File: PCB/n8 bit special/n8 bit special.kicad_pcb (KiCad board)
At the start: 4 copper layers, 99.9 x 100 mm, 50 parts, among them J1 USB_B_Micro, J2 PORT0, J3 PORT2, J4 PORT1, J6 Conn_02x08_Odd_Even, Q1 2N3904, SW1 SW_Push_Dual, U1 W65C02SxP, U10 74HC00, U2 CY62256-70PC, U3 CY62256-70PC, U4 28C256, U5 74LS21, U6 22V10C, U7 DS1813, U8 SC28L92_PLC44, U9 FT230XS, X1 3.6864Mhz

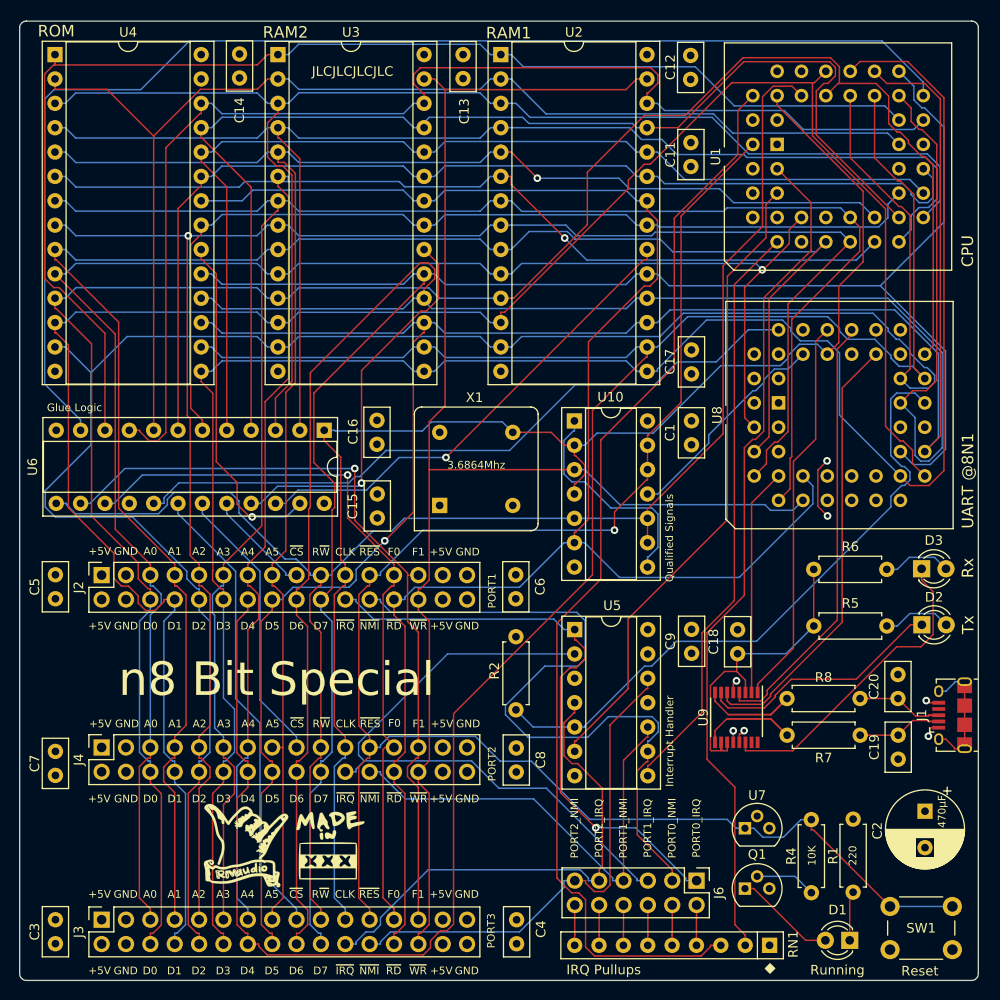
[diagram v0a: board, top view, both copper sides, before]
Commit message: release candidate for v2
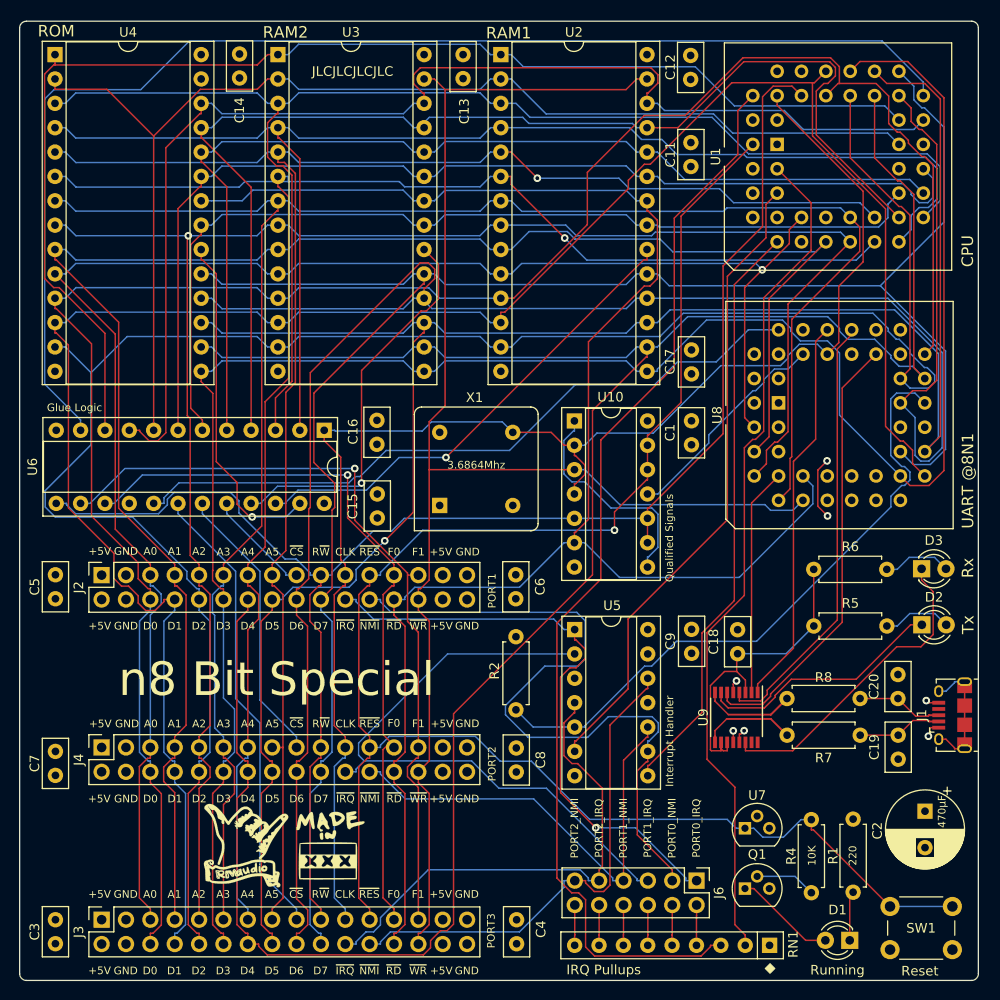
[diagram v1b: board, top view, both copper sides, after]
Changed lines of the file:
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@@
-(kicad_pcb (version 20171130) (host pcbnew "(5.1.9-0-10_14)")
+(kicad_pcb (version 20171130) (host pcbnew "(5.1.12-1-10_14)")
   (general
     (thickness 1.6)
@@
     )
   )
+  (gr_text GND (at 133.60908 130.90652) (layer F.SilkS)
+    (effects (font (size 0.8 0.8) (thickness 0.15)))
+  )
+  (gr_text ~RES (at 123.44908 130.90652) (layer F.SilkS)
+    (effects (font (size 0.8 0.8) (thickness 0.15)))
+  )
+  (gr_text +5V (at 130.89128 130.89382) (layer F.SilkS)
+    (effects (font (size 0.8 0.8) (thickness 0.15)))
+  )
+  (gr_text R~W (at 118.36908 130.90652) (layer F.SilkS)
+    (effects (font (size 0.8 0.8) (thickness 0.15)))
+  )
+  (gr_text A0 (at 100.58908 130.90652) (layer F.SilkS)
+    (effects (font (size 0.8 0.8) (thickness 0.15)))
+  )
+  (gr_text GND (at 98.04908 130.90652) (layer F.SilkS)
+    (effects (font (size 0.8 0.8) (thickness 0.15)))
+  )
+  (gr_text A2 (at 105.66908 130.90652) (layer F.SilkS)
+    (effects (font (size 0.8 0.8) (thickness 0.15)))
+  )
+  (gr_text +5V (at 95.33128 130.90652) (layer F.SilkS)
+    (effects (font (size 0.8 0.8) (thickness 0.15)))
+  )
+  (gr_text A1 (at 103.12908 130.90652) (layer F.SilkS)
+    (effects (font (size 0.8 0.8) (thickness 0.15)))
+  )
+  (gr_text F1 (at 128.52908 130.90652) (layer F.SilkS)
+    (effects (font (size 0.8 0.8) (thickness 0.15)))
+  )
+  (gr_text CLK (at 120.90908 130.90652) (layer F.SilkS)
+    (effects (font (size 0.8 0.8) (thickness 0.15)))
+  )
+  (gr_text F0 (at 125.98908 130.90652) (layer F.SilkS)
+    (effects (font (size 0.8 0.8) (thickness 0.15)))
+  )
+  (gr_text A3 (at 108.20908 130.90652) (layer F.SilkS)
+    (effects (font (size 0.8 0.8) (thickness 0.15)))
+  )
+  (gr_text ~CS (at 115.82908 130.90652) (layer F.SilkS)
+    (effects (font (size 0.8 0.8) (thickness 0.15)))
+  )
+  (gr_text A5 (at 113.28908 130.90652) (layer F.SilkS)
+    (effects (font (size 0.8 0.8) (thickness 0.15)))
+  )
+  (gr_text "A4\n" (at 110.74908 130.90652) (layer F.SilkS)
+    (effects (font (size 0.8 0.8) (thickness 0.15)))
+  )
   (gr_text JLCJLCJLCJLC (at 121.7041 45.1231) (layer F.SilkS)
     (effects (font (size 1 1) (thickness 0.15)))
@@
   (gr_arc (start 87.6935 139.192) (end 86.995 139.192) (angle -90) (layer Edge.Cuts) (width 0.1))
   (gr_arc (start 186.2455 139.192) (end 186.2455 139.8905) (angle -90) (layer Edge.Cuts) (width 0.1))
-  (gr_arc (start 87.6935 40.5765) (end 87.6935 39.878) (angle -90) (layer Edge.Cuts) (width 0.1))
-  (gr_arc (start 186.2455 40.5765) (end 186.944 40.5765) (angle -90) (layer Edge.Cuts) (width 0.1))
+  (gr_arc (start 87.6935 40.5892) (end 87.6935 39.8907) (angle -90) (layer Edge.Cuts) (width 0.1))
+  (gr_arc (start 186.2455 40.5892) (end 186.944 40.5892) (angle -90) (layer Edge.Cuts) (width 0.1))
   (gr_text 220 (at 173.8503 126.873 90) (layer F.SilkS)
     (effects (font (size 0.8 0.8) (thickness 0.15)))
@@
     (effects (font (size 0.8 0.8) (thickness 0.15)))
   )
-  (gr_text GND (at 133.60908 130.90652) (layer F.SilkS)
-    (effects (font (size 0.8 0.8) (thickness 0.15)))
-  )
-  (gr_text ~RES (at 123.44908 130.90652) (layer F.SilkS)
-    (effects (font (size 0.8 0.8) (thickness 0.15)))
-  )
-  (gr_text +5V (at 130.89128 130.89382) (layer F.SilkS)
-    (effects (font (size 0.8 0.8) (thickness 0.15)))
-  )
-  (gr_text R~W (at 118.36908 130.90652) (layer F.SilkS)
-    (effects (font (size 0.8 0.8) (thickness 0.15)))
-  )
-  (gr_text A0 (at 100.58908 130.90652) (layer F.SilkS)
-    (effects (font (size 0.8 0.8) (thickness 0.15)))
-  )
-  (gr_text GND (at 98.04908 130.90652) (layer F.SilkS)
-    (effects (font (size 0.8 0.8) (thickness 0.15)))
-  )
-  (gr_text A2 (at 105.66908 130.90652) (layer F.SilkS)
-    (effects (font (size 0.8 0.8) (thickness 0.15)))
-  )
-  (gr_text +5V (at 95.33128 130.90652) (layer F.SilkS)
-    (effects (font (size 0.8 0.8) (thickness 0.15)))
-  )
-  (gr_text A1 (at 103.12908 130.90652) (layer F.SilkS)
-    (effects (font (size 0.8 0.8) (thickness 0.15)))
-  )
-  (gr_text F1 (at 128.52908 130.90652) (layer F.SilkS)
-    (effects (font (size 0.8 0.8) (thickness 0.15)))
-  )
-  (gr_text CLK (at 120.90908 130.90652) (layer F.SilkS)
-    (effects (font (size 0.8 0.8) (thickness 0.15)))
-  )
-  (gr_text F0 (at 125.98908 130.90652) (layer F.SilkS)
-    (effects (font (size 0.8 0.8) (thickness 0.15)))
-  )
-  (gr_text A3 (at 108.20908 130.90652) (layer F.SilkS)
-    (effects (font (size 0.8 0.8) (thickness 0.15)))
-  )
-  (gr_text ~CS (at 115.82908 130.90652) (layer F.SilkS)
-    (effects (font (size 0.8 0.8) (thickness 0.15)))
-  )
-  (gr_text A5 (at 113.28908 130.90652) (layer F.SilkS)
-    (effects (font (size 0.8 0.8) (thickness 0.15)))
-  )
-  (gr_text "A4\n" (at 110.74908 130.90652) (layer F.SilkS)
-    (effects (font (size 0.8 0.8) (thickness 0.15)))
-  )
-  (gr_text GND (at 133.75386 113.1316) (layer F.SilkS)
+  (gr_text GND (at 133.6675 113.1189) (layer F.SilkS)
     (effects (font (size 0.8 0.8) (thickness 0.15)))
   )
-  (gr_text ~RES (at 123.53036 113.1316) (layer F.SilkS)
+  (gr_text ~RES (at 123.4821 113.1316) (layer F.SilkS)
     (effects (font (size 0.8 0.8) (thickness 0.15)))
   )
@@
     (effects (font (size 0.8 0.8) (thickness 0.15)))
   )
-  (gr_text R~W (at 118.45036 113.1316) (layer F.SilkS)
+  (gr_text R~W (at 118.4148 113.1316) (layer F.SilkS)
     (effects (font (size 0.8 0.8) (thickness 0.15)))
   )
@@
     (effects (font (size 0.8 0.8) (thickness 0.15)))
   )
-  (gr_text A2 (at 105.75036 113.1316) (layer F.SilkS)
+  (gr_text A2 (at 105.7021 113.1316) (layer F.SilkS)
     (effects (font (size 0.8 0.8) (thickness 0.15)))
   )
@@
     (effects (font (size 0.8 0.8) (thickness 0.15)))
   )
-  (gr_text A1 (at 103.21036 113.1316) (layer F.SilkS)
+  (gr_text A1 (at 103.1494 113.1316) (layer F.SilkS)
     (effects (font (size 0.8 0.8) (thickness 0.15)))
   )
-  (gr_text F1 (at 128.61036 113.1316) (layer F.SilkS)
+  (gr_text F1 (at 128.5621 113.1189) (layer F.SilkS)
     (effects (font (size 0.8 0.8) (thickness 0.15)))
   )
-  (gr_text CLK (at 120.99036 113.1316) (layer F.SilkS)
+  (gr_text CLK (at 120.9675 113.1316) (layer F.SilkS)
     (effects (font (size 0.8 0.8) (thickness 0.15)))
   )
-  (gr_text F0 (at 126.07036 113.0681) (layer F.SilkS)
+  (gr_text F0 (at 126.0094 113.0681) (layer F.SilkS)
     (effects (font (size 0.8 0.8) (thickness 0.15)))
   )
-  (gr_text A3 (at 108.29036 113.1316) (layer F.SilkS)
+  (gr_text A3 (at 108.2548 113.1316) (layer F.SilkS)
     (effects (font (size 0.8 0.8) (thickness 0.15)))
   )
-  (gr_text ~CS (at 115.91036 113.1316) (layer F.SilkS)
+  (gr_text ~CS (at 115.8621 113.1316) (layer F.SilkS)
     (effects (font (size 0.8 0.8) (thickness 0.15)))
   )
-  (gr_text A5 (at 113.37036 113.1316) (layer F.SilkS)
+  (gr_text A5 (at 113.3348 113.1316) (layer F.SilkS)
     (effects (font (size 0.8 0.8) (thickness 0.15)))
   )
-  (gr_text "A4\n" (at 110.83036 113.1316) (layer F.SilkS)
+  (gr_text "A4\n" (at 110.7821 113.1316) (layer F.SilkS)
     (effects (font (size 0.8 0.8) (thickness 0.15)))
   )
@@
     (effects (font (size 0.8 0.8) (thickness 0.15)))
   )
-  (gr_line (start 186.944 40.5765) (end 186.944 139.192) (layer Edge.Cuts) (width 0.1))
-  (gr_line (start 87.6935 39.878) (end 186.2455 39.878) (layer Edge.Cuts) (width 0.1))
-  (gr_line (start 86.995 139.192) (end 86.995 40.5765) (layer Edge.Cuts) (width 0.1))
+  (gr_line (start 186.944 40.5892) (end 186.944 139.192) (layer Edge.Cuts) (width 0.1))
+  (gr_line (start 87.6935 39.8907) (end 186.2455 39.8907) (layer Edge.Cuts) (width 0.1))
+  (gr_line (start 86.995 139.192) (end 86.995 40.5892) (layer Edge.Cuts) (width 0.1))
   (gr_line (start 186.2455 139.8905) (end 87.6935 139.8905) (layer Edge.Cuts) (width 0.1))
   (dimension 100.012501 (width 0.15) (layer Dwgs.User)
